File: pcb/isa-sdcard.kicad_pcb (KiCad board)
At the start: 2 copper layers, 123.7 x 73 mm, 34 parts, among them J1 SD Card Board, J3 Bus_ISA_8bit_AB_Rev0, SW1 ADDR SEL, U10 74HC32, U12 74HC165, U13 74HC595, U14 74HC00, U2 74HC00, U22 74HCT688, U4 74HC00, U5 74HC163, U6 74HCT138, U7 74HC123, U9 74HC32, X1 16MHz

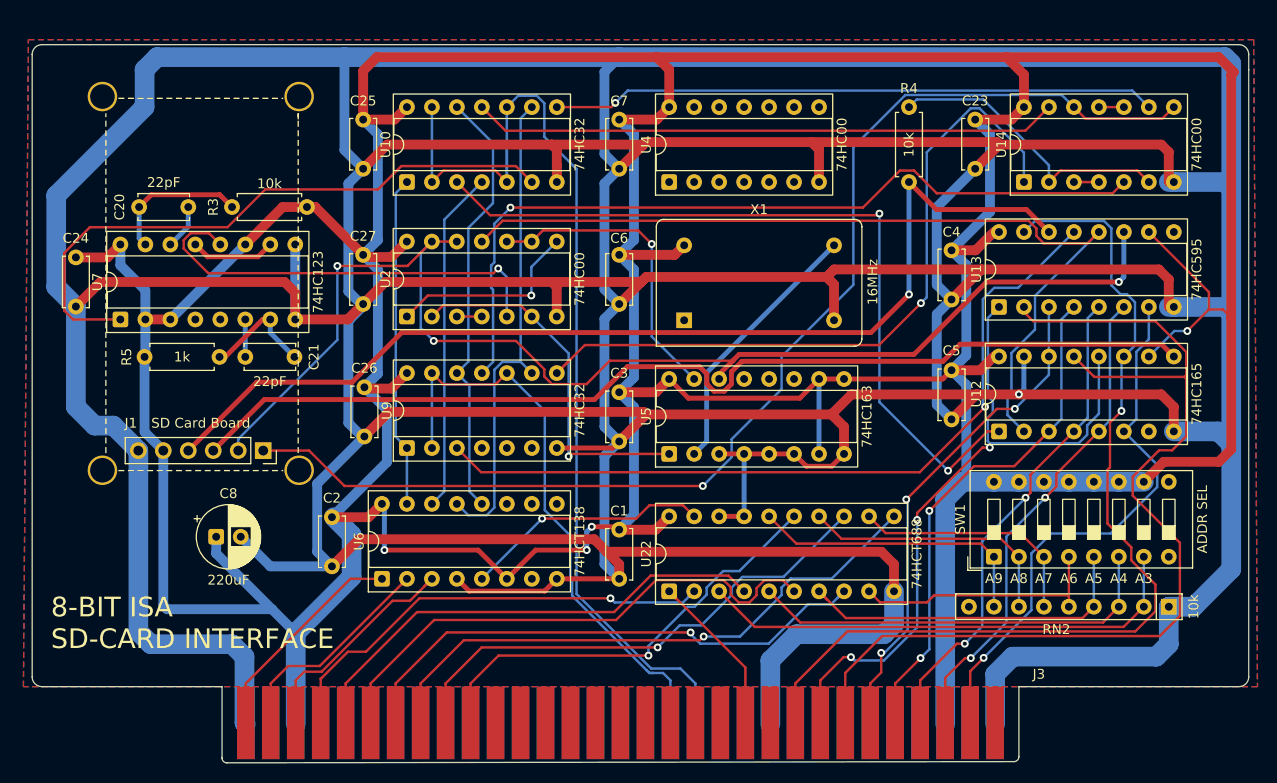
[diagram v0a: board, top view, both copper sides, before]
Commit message: Revising schematics and layout
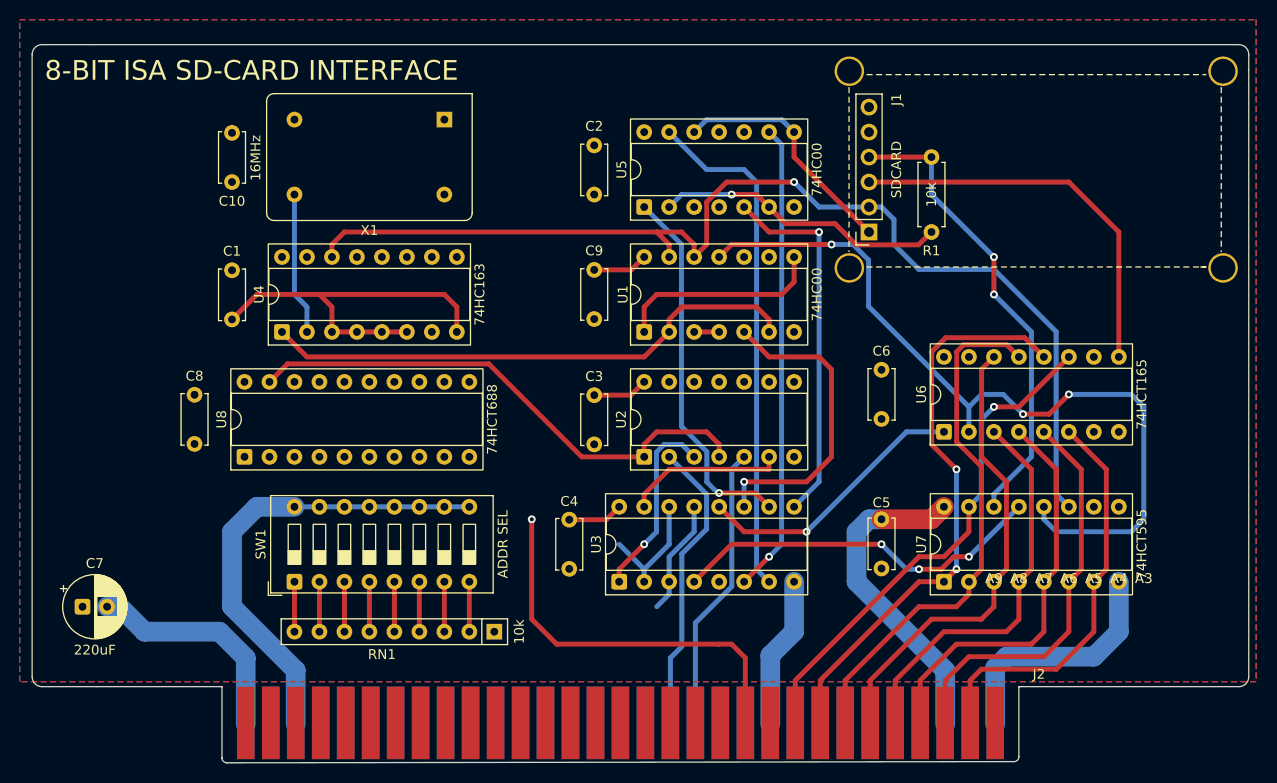
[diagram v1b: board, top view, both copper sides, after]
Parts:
- removed the C1 at (117.1, 101.5)
- removed C20, C21: 22pF, Capacitor_THT:C_Disc_D5.0mm_W2.5mm_P5.00mm
- removed C25: 0.1uF, Capacitor_THT:C_Disc_D5.0mm_W2.5mm_P5.00mm
- removed the C5 at (150.9, 85.3)
- removed R3: 10k, Resistor_THT:R_Axial_DIN0207_L6.3mm_D2.5mm_P7.62mm_Horizontal
- removed R5: 1k, Resistor_THT:R_Axial_DIN0207_L6.3mm_D2.5mm_P7.62mm_Horizontal
- removed U10, U9: 74HC32, Package_DIP:DIP-14_W7.62mm_Socket
- removed the U4 at (122.2, 61.2)
- removed the U6 at (93.0, 101.5)
- removed the U7 at (66.4, 75.2)
- added U2: 74HCT32, Package_DIP:DIP-14_W7.62mm_Socket, F.Cu at (119.6, 89.1)
- added U3: 74HCT139, Package_DIP:DIP-16_W7.62mm_Socket, F.Cu at (117.1, 101.8)
- J1: value SD Card Board -> SDCARD
- U6: renamed from U12; value 74HC165 -> 74HCT165
- U7: renamed from U13; value 74HC595 -> 74HCT595
- moved SW1 71.2 mm to (84.1, 101.8)
- moved RN1 68.6 mm to (104.4, 106.9)
- moved J1 65.5 mm to (142.5, 66.3), turned to 180 degrees
- moved C3 47.8 mm to (114.5, 87.9)
- moved C4 47.5 mm to (112.0, 100.5)
- moved U8 45.3 mm to (79.0, 89.1)
- moved U4 41.3 mm to (82.8, 76.4)
- moved U5 38.7 mm to (119.6, 63.7)
- moved C5 37.9 mm to (143.7, 100.5)
- moved C6 36.9 mm to (143.7, 85.3)
- moved X1 31.8 mm to (99.3, 54.9), turned to 180 degrees
- moved U7 28.5 mm to (150.1, 101.8)
- moved C1 27.1 mm to (77.7, 75.2)
- moved C9 26.2 mm to (114.5, 75.1)
- moved C2 25.2 mm to (114.5, 62.5)
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- renumbered C2 to C1, C24 to C10, C3 to C2, C23 to C3, C6 to C5, C7 to C6, C8 to C7, C27 to C8, C26 to C9, J3 to J2, R4 to R1, RN2 to RN1, U2 to U1, U5 to U4, U14 to U5, U22 to U8
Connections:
- net SD_SPI renamed Net-(U4-~{MR})
- C1 pad 2: +5V -> VCC
- C10 pad 1: +5V -> VCC
- C2 pad 2: +5V -> VCC
- C3 pad 2: +5V -> VCC
- C4 pad 2: +5V -> VCC
- C5 pad 2: +5V -> VCC
- C6 pad 2: +5V -> VCC
- C7 pad 1: +5V -> VCC
- C8 pad 2: +5V -> VCC
- C9 pad 2: +5V -> VCC
- J1 pad 5: +5V -> VCC
- J2 pad B02: RESET -> unconnected-(J2-RESET-PadB02)
- J2 pad B03: +5V -> VCC
- J2 pad B29: +5V -> VCC
- RN1 pad 2: Net-(RN2-R1) -> Net-(RN1-R1)
- RN1 pad 3: Net-(RN2-R2) -> Net-(RN1-R2)
- RN1 pad 4: Net-(RN2-R3) -> Net-(RN1-R3)
- RN1 pad 5: Net-(RN2-R4) -> Net-(RN1-R4)
- RN1 pad 6: Net-(RN2-R5) -> Net-(RN1-R5)
- RN1 pad 7: Net-(RN2-R6) -> Net-(RN1-R6)
- RN1 pad 8: Net-(RN2-R7) -> Net-(RN1-R7)
- RN1 pad 9: unconnected-(RN2-R8-Pad9) -> Net-(RN1-R8)
- SW1 pad 1: Net-(RN2-R7) -> Net-(RN1-R8)
- SW1 pad 10: +5V -> VCC
- SW1 pad 11: +5V -> VCC
- SW1 pad 12: +5V -> VCC
- SW1 pad 13: +5V -> VCC
- SW1 pad 14: +5V -> VCC
- SW1 pad 15: +5V -> VCC
- SW1 pad 16: +5V -> VCC
- SW1 pad 2: Net-(RN2-R6) -> Net-(RN1-R7)
- SW1 pad 3: Net-(RN2-R5) -> Net-(RN1-R6)
- SW1 pad 4: Net-(RN2-R4) -> Net-(RN1-R5)
- SW1 pad 5: Net-(RN2-R3) -> Net-(RN1-R4)
- SW1 pad 6: Net-(RN2-R2) -> Net-(RN1-R3)
- SW1 pad 7: Net-(RN2-R1) -> Net-(RN1-R2)
- SW1 pad 8: unconnected-(SW1-Pad8) -> Net-(RN1-R1)
- SW1 pad 9: unconnected-(SW1-Pad9) -> VCC
- U1 pad 14: +5V -> VCC
- U1 pad 5: ~{CLKSTART_DB} -> ~{CLKSTART}
- U4 pad 10: +5V -> VCC
- U4 pad 16: +5V -> VCC
- U4 pad 7: +5V -> VCC
- U4 pad 9: +5V -> VCC
- U5 pad 14: +5V -> VCC
- U6 pad 10: +5V -> VCC
- U6 pad 16: +5V -> VCC
- U7 pad 10: +5V -> VCC
- U7 pad 16: +5V -> VCC
- U8 pad 11: A7 -> A6
- U8 pad 12: Net-(RN2-R5) -> Net-(RN1-R5)
- U8 pad 13: A8 -> A7
- U8 pad 14: Net-(RN2-R6) -> Net-(RN1-R6)
- U8 pad 15: A9 -> A8
- U8 pad 16: Net-(RN2-R7) -> Net-(RN1-R7)
- U8 pad 17: GND -> A9
- U8 pad 18: GND -> Net-(RN1-R8)
- U8 pad 2: A3 -> A2
- U8 pad 20: +5V -> VCC
- U8 pad 3: Net-(RN2-R1) -> Net-(RN1-R1)
- U8 pad 4: A4 -> A3
- U8 pad 5: Net-(RN2-R2) -> Net-(RN1-R2)
- U8 pad 6: A5 -> A4
- U8 pad 7: Net-(RN2-R3) -> Net-(RN1-R3)
- U8 pad 8: A6 -> A5
- U8 pad 9: Net-(RN2-R4) -> Net-(RN1-R4)
- X1 pad 14: +5V -> VCC
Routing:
- net GND: track 945.0 -> 102.3 mm, vias 1 -> 0
- net +5V: track 607.5 -> 0.00 mm, vias 4 -> 0
- net ~{CS}: track 124.5 -> 24.5 mm, vias 1 -> 0
- net VCC: track 0.00 -> 97.5 mm
- net ~{WR}: track 103.5 -> 29.2 mm
- net MOSI: track 106.5 -> 40.2 mm
- net MISO: track 107.6 -> 47.7 mm, vias 1 -> 2
- net A7: track 59.7 -> 0.00 mm, vias 1 -> 0
- net A6: track 55.6 -> 0.00 mm, vias 1 -> 0
- net A5: track 55.5 -> 0.00 mm
- net ~{SER_WR}: track 80.3 -> 28.1 mm, vias 2 -> 1
- net A8: track 52.1 -> 0.00 mm, vias 1 -> 0
- net D2: track 105.2 -> 54.0 mm
- net A4: track 50.7 -> 0.00 mm
- net Net-(RN2-R1): track 50.6 -> 0.00 mm
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- added copper zone on B.Cu, net VCC
- removed copper zone on B.Cu, net GND
